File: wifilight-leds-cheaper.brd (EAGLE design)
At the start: 50.8 x 50.8 mm, 55 parts, among them Q1 BUK98180-100A, Q2 BUK98180-100A, Q3 BUK98180-100A, Q4 BUK98180-100A, U2 PCA9685

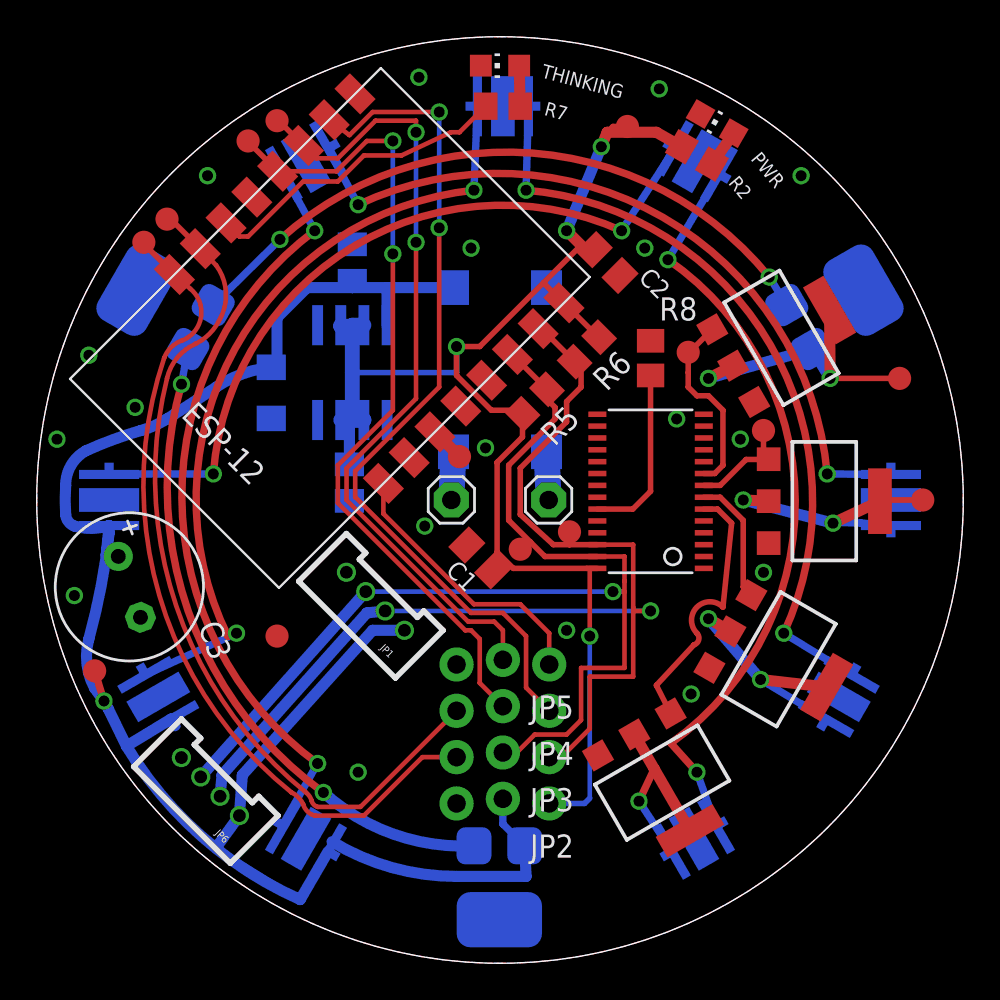
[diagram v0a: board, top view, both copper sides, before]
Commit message: Mk6 complete & DRC'd
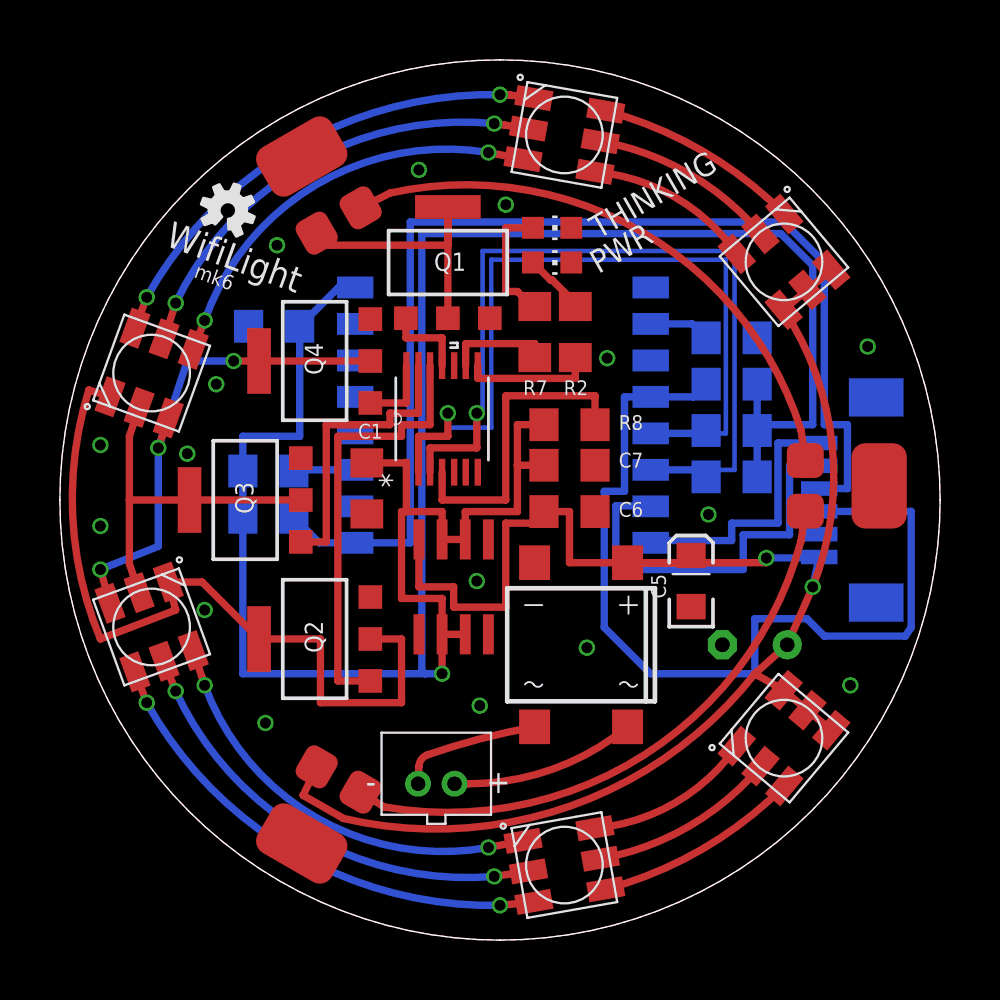
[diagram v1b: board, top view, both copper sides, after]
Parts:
- removed A, B: (no value), adafruit:1X01
- removed JP1, JP6: (no value), SparkFun-Connectors:1X04-1.5MM_JST
- removed JP2, JP3, JP4, JP5: (no value), SparkFun-Connectors:1X03_LOCK_NO_SILK
- removed LB1, LB2, LB3, LG1, LG2, LG3, LR1, LR2, LR3: XPEWHT-01-0000-00BC2, led:CREE_XLAMP
- removed P_RED, P_WHITE, RED, SCL, SDA, TP12V, TP3.3V, TPCHPD, TPGND, TPGPIO0, TPGPIO2, TPRX, TPTX, WHITE: TEST-POINT3X5, SparkFun-Passives:PAD.03X.05
- removed U2: PCA9685, adafruit:TSSOP28
- added CN1: (no value), adafruit:JST-PH-2-THM
- added LED1, LED2, LED3, LED4, LED5, LED6: RGBLED5050, adafruit:RGBLED5050
- added R10, R11, R12, R13: 10k, SparkFun-Resistors:1206
- added U$2: (no value), SparkFun-Aesthetics:OSHW-LOGO-S
- added U1: TCA6507PW, Texas Instruments_By_element14_Batch_1:SOP65P640X120-14N
- added X1: 53261-06, con-molex:53261-06
- C1, C2, C6, C7: device resistor:C0805K -> SparkFun-Passives:1206
- R2, R7: value ??? -> 220ohm; device resistor:R0805 -> SparkFun-Passives:1206
- R5, R6, R8: device resistor:R0805 -> SparkFun-Passives:1206
- moved WL2 39.4 mm to (44.8, 26.2), flipped to the top, turned to 90 degrees
- moved C3 34.4 mm to (39.4, 17.5), flipped to the bottom, turned to 0 degrees
- moved Q3 31.8 mm to (11.4, 25.4), turned to 90 degrees
- moved Q4 30.2 mm to (15.2, 33.0), turned to 90 degrees
- moved WL1 29.6 mm to (15.2, 43.0), flipped to the top, turned to 210 degrees
- moved C5 25.2 mm to (35.9, 21.0), flipped to the top
- moved Q2 20.6 mm to (15.2, 17.8), turned to 90 degrees
- moved Q1 18.7 mm to (22.5, 38.4), turned to 0 degrees
- moved C2 18.6 mm to (13.0, 34.9), flipped to the bottom, turned to 0 degrees
- moved C6 18.1 mm to (29.2, 24.8), flipped to the top, turned to 0 degrees
- moved B2 15.7 mm to (29.8, 17.5), flipped to the top
- moved REG2 13.0 mm to (22.9, 20.6), flipped to the top
- moved MPU 12.9 mm to (17.5, 39.1), flipped to the bottom, turned to 180 degrees
- moved R7 12.5 mm to (27.3, 34.6), turned to 90 degrees
- moved C7 12.1 mm to (29.2, 27.3), flipped to the top, turned to 0 degrees
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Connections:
- net N$25 renamed GPIO14
- net N$26 renamed GPIO16
- net N$28 renamed ADC
- removed net #OE: R8.2, U2.23
- removed net B1: LB2.A, LB2.A@1, LB3.C, LB3.C@1
- removed net B2: LB1.A, LB1.A@1, LB2.C, LB2.C@1
- removed net G1: LG2.A, LG2.A@1, LG3.C, LG3.C@1
- removed net G2: LG1.A, LG1.A@1, LG2.C, LG2.C@1
- removed net N$18: A.1, B2.AC1
- removed net N$19: B.1, B2.AC2
- removed net N$36: MPU.5
- removed net R1: LR2.A, LR2.A@1, LR3.C, LR3.C@1
- removed net R2: LR1.A, LR1.A@1, LR2.C, LR2.C@1
- new net AC1: B2.AC1, CN1.1
- new net AC2: B2.AC2, CN1.2
- new net EN: R8.2, U1.4
- new net GPIO12: MPU.14
- new net GPIO13: MPU.15
- new net N$30: LED2.5, LED3.2
- new net N$31: LED2.6, LED3.1
- new net N$32: LED2.4, LED3.3
- new net N$33: LED1.5, LED2.2
- new net N$34: LED1.6, LED2.1
- new net N$35: LED1.4, LED2.3
- new net N$37: LED4.5, LED5.2
- new net N$38: LED4.6, LED5.1
- new net N$39: LED4.4, LED5.3
- new net N$40: LED5.5, LED6.2
- new net N$41: LED5.6, LED6.1
- new net N$42: LED5.4, LED6.3
- new net N$6: U1.10
- new net POWERED: R2.1, U1.8
- net 12V: now also LED1.1, LED1.2, LED1.3, LED4.1, LED4.2, LED4.3, X1.6; no longer JP1.1, JP2.2, JP6.1, LB3.A, LB3.A@1, LG3.A, LG3.A@1, LR3.A, LR3.A@1, TP12V.P$1
- net 3.3V: now also R10.1, R11.1, R12.1, R8.1, U1.1; no longer JP2.1, R2.1, TP3.3V.P$1, U2.28
- net BLUE: now also U1.12; no longer U2.6
- net CH_PD: now also R11.2; no longer TPCHPD.P$1
- net GND: now also R13.1, U1.5, U1.6, U1.7, X1.5; no longer JP1.4, JP2.3, JP5.3, JP6.4, R8.1, TPGND.P$1, U2.14, U2.25
- net GPIO0: now also R12.2, X1.4; no longer JP4.2, TPGPIO0.P$1
- net GPIO15: now also R13.2; no longer JP4.1
- net GPIO2: no longer JP5.2, TPGPIO2.P$1
- net GREEN: now also U1.14; no longer U2.7
- net P_BLUE: now also LED3.4, LED6.4; no longer LB1.C, LB1.C@1
- net P_GREEN: now also LED3.6, LED6.6; no longer LG1.C, LG1.C@1
- net P_RED: now also LED3.5, LED6.5; no longer LR1.C, LR1.C@1, P_RED.P$1
- net P_WHITE: no longer P_WHITE.P$1
- net RED: now also U1.13; no longer RED.P$1, U2.8
- net RESET: now also R10.2, X1.3; no longer JP5.1
- net RXD: now also X1.2; no longer JP4.3, TPRX.P$1
- net SCL: now also MPU.5, U1.2; no longer JP1.2, JP3.1, JP6.2, MPU.15, SCL.P$1, U2.26
- net SDA: now also MPU.6, U1.3; no longer JP1.3, JP3.2, JP6.3, MPU.14, SDA.P$1, U2.27
- net THINKING: now also U1.9; no longer MPU.6
- net TXD: now also X1.1; no longer JP3.3, TPTX.P$1
- net WHITE: now also U1.11; no longer U2.9, WHITE.P$1
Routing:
- net 3.3V: track 81.4 -> 134.5 mm, vias 4 -> 1
- net RESET: track 15.2 -> 63.4 mm
- net GPIO2: track 44.9 -> 0.00 mm, vias 2 -> 0
- net GPIO15: track 47.0 -> 3.35 mm, vias 2 -> 0
- net G1: track 39.4 -> 0.00 mm, vias 2 -> 0
- net B2: track 38.1 -> 0.00 mm, vias 2 -> 0
- net B1: track 38.0 -> 0.00 mm, vias 2 -> 0
- net G2: track 37.9 -> 0.00 mm, vias 2 -> 0
- net R1: track 37.8 -> 0.00 mm, vias 2 -> 0
- net R2: track 37.5 -> 0.00 mm, vias 2 -> 0
- net P_BLUE: track 11.8 -> 43.7 mm, vias 1 -> 0
- net TXD: track 43.6 -> 14.7 mm
- net N$42: track 0.00 -> 26.6 mm, vias 0 -> 2
- net N$31: track 0.00 -> 26.0 mm, vias 0 -> 2
- net N$40: track 0.00 -> 24.0 mm, vias 0 -> 2
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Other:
- board size 50.8 x 50.8 mm -> 48.3 x 48.3 mm
- board text added: "WifiLight"
- board text added: "mk6"
